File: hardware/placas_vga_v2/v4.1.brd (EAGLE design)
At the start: 32 x 39.9 mm, 39 parts

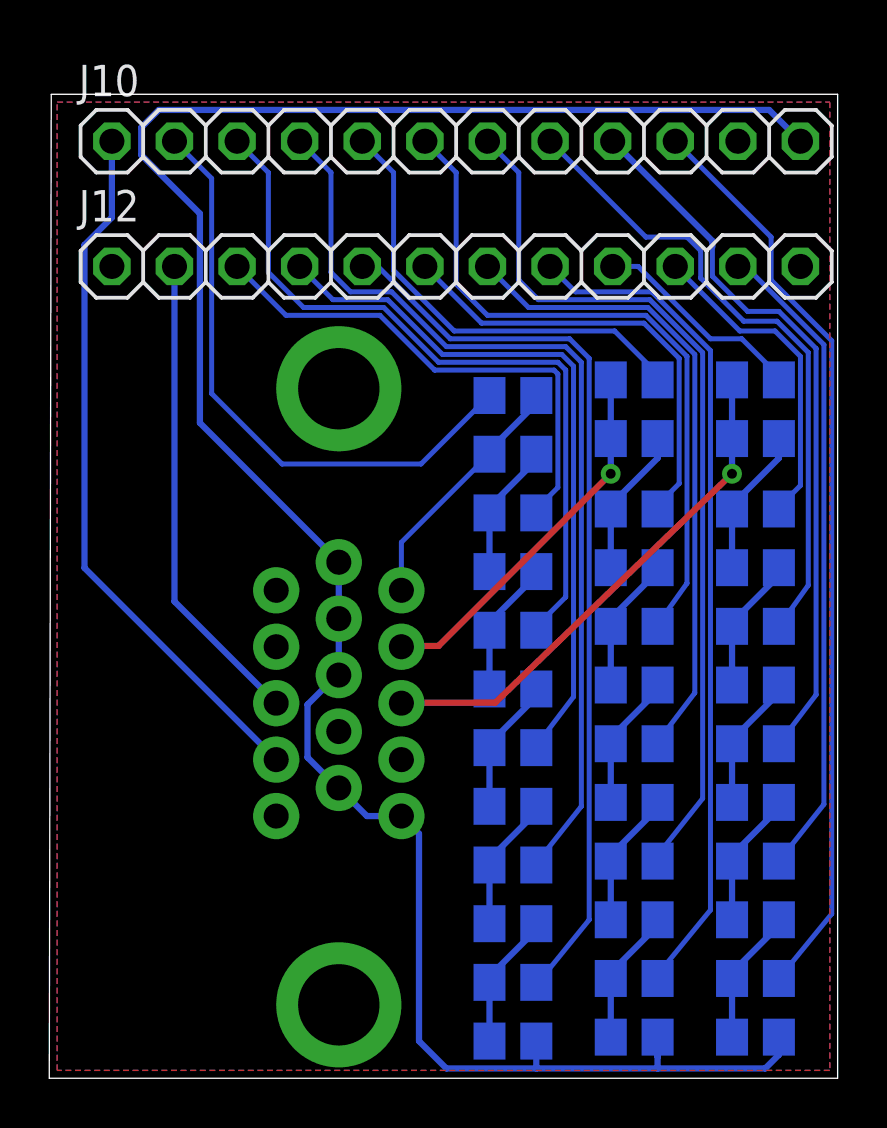
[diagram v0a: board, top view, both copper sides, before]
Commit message: Actualizo varios
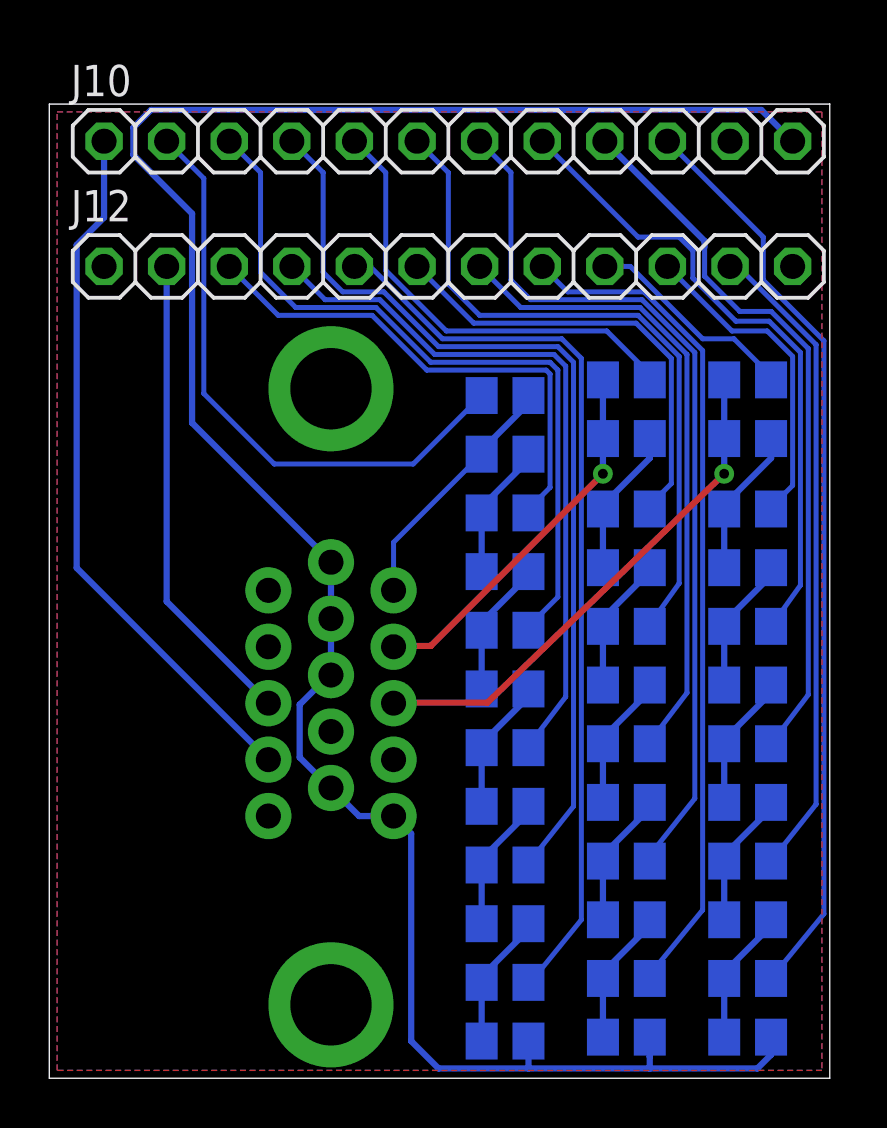
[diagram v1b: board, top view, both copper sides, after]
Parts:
- moved J10 0.32 mm to (16.2, 38.0)
- moved J12 0.32 mm to (16.2, 32.9)
- moved R10 0.32 mm to (23.4, 18.3)
- moved R11 0.32 mm to (23.4, 13.6)
- moved R12 0.32 mm to (23.4, 8.81)
- moved R13 0.32 mm to (23.4, 4.05)
- moved R14 0.32 mm to (23.4, 1.67)
- moved R15 0.32 mm to (28.3, 28.3)
- moved R16 0.32 mm to (28.3, 23.1)
- moved R17 0.32 mm to (28.3, 18.3)
- moved R18 0.32 mm to (28.3, 13.6)
- moved R19 0.32 mm to (28.3, 8.81)
- moved R20 0.32 mm to (28.3, 4.05)
- moved R21 0.32 mm to (28.3, 1.67)
- moved R27 0.32 mm to (23.4, 26.0)
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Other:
- board size 32 x 39.9 mm -> 31.7 x 39.5 mm
